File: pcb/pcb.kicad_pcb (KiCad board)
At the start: 2 copper layers, 49 x 31 mm, 35 parts, among them J1 Conn_02x08_Odd_Even, J2 B2B-PH-K-S_LF__SN_, J3 USB_C_Receptacle, Q1 MMUN2211LT1G, SW1 SW_SPST, U1 TPS61090, U2 MCP73871-1AA

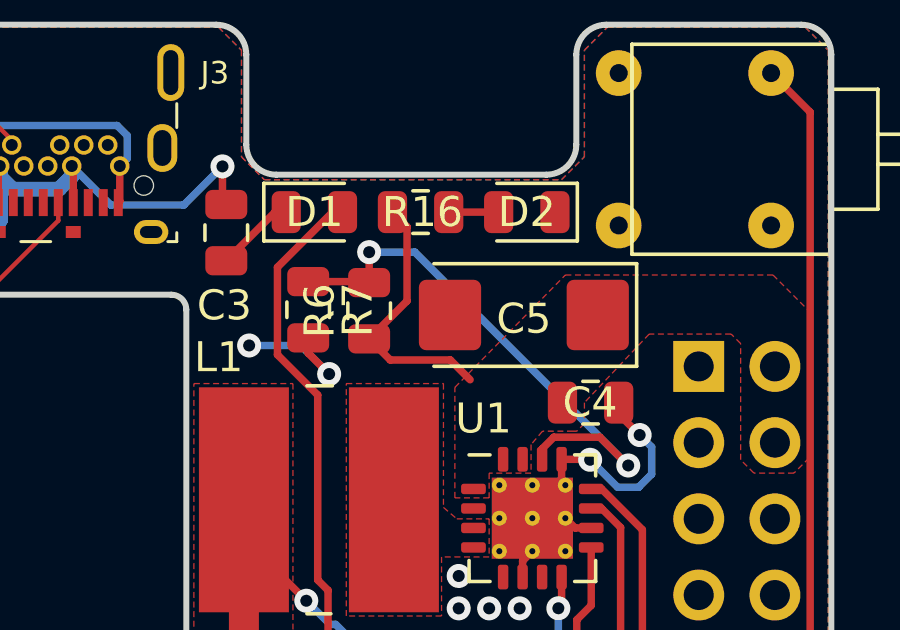
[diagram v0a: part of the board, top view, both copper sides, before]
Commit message: updated schematic
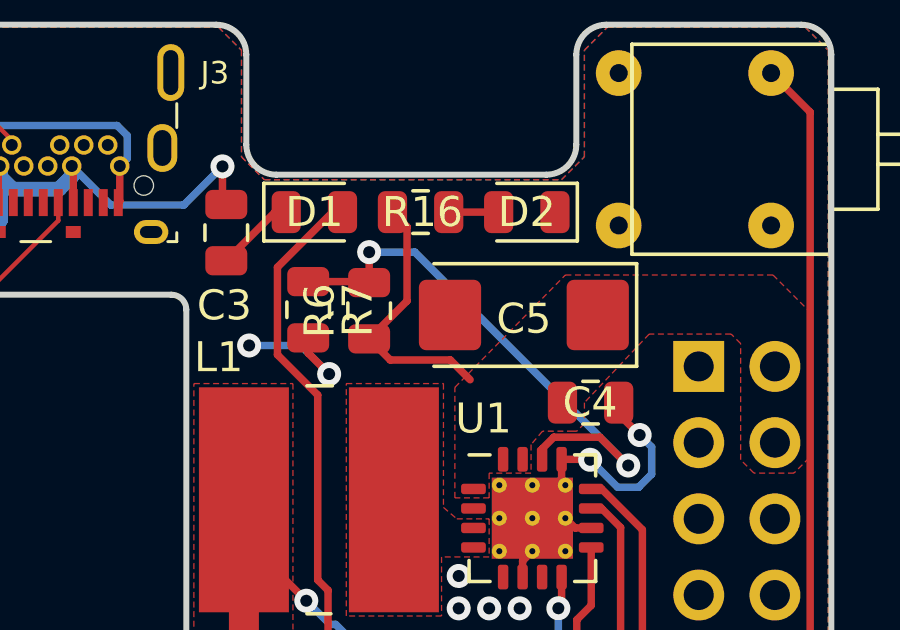
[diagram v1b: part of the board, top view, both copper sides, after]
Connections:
- D3 pad 1: VBUS -> Net-(D3-Pad1)
- D3 pad 2: Net-(D3-Pad2) -> VBUS
- D4 pad 1: VBUS -> Net-(D4-Pad1)
- D4 pad 2: Net-(D4-Pad2) -> VBUS
- J1 pad 6: Net-(J1-Pad6) -> GND
- R13 pad 1: Net-(D3-Pad2) -> Net-(D3-Pad1)
- R14 pad 1: Net-(D4-Pad2) -> Net-(D4-Pad1)
